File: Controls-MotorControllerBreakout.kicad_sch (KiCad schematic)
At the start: 12 parts, among them J1 MC CAN 1, J2 MC CAN 2, J3 CTRLS, J4 EXT PWR, J5 CANDAPTER

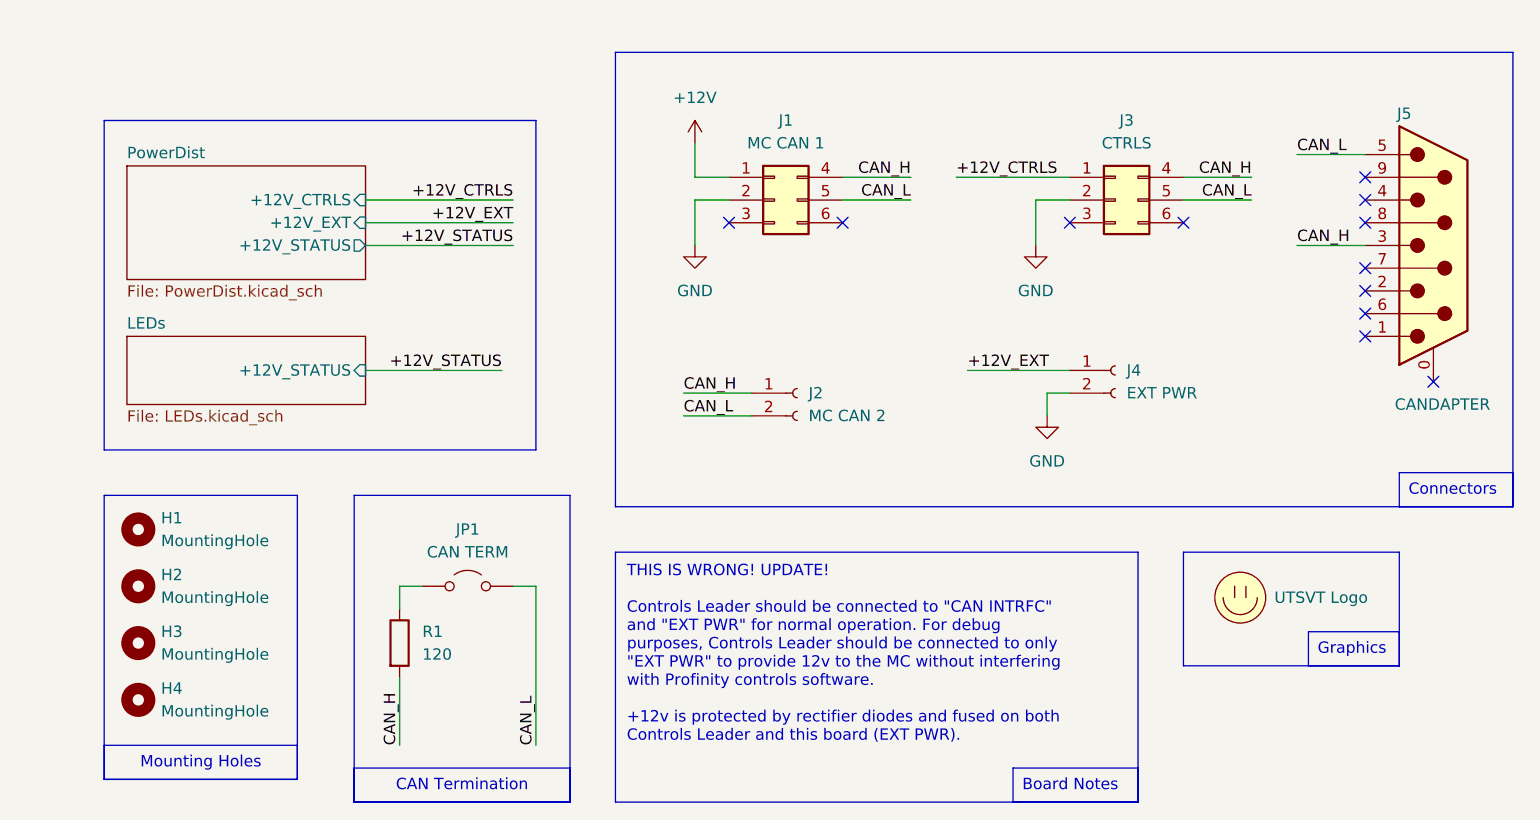
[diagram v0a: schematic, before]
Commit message: layout kinda screwy but it works?
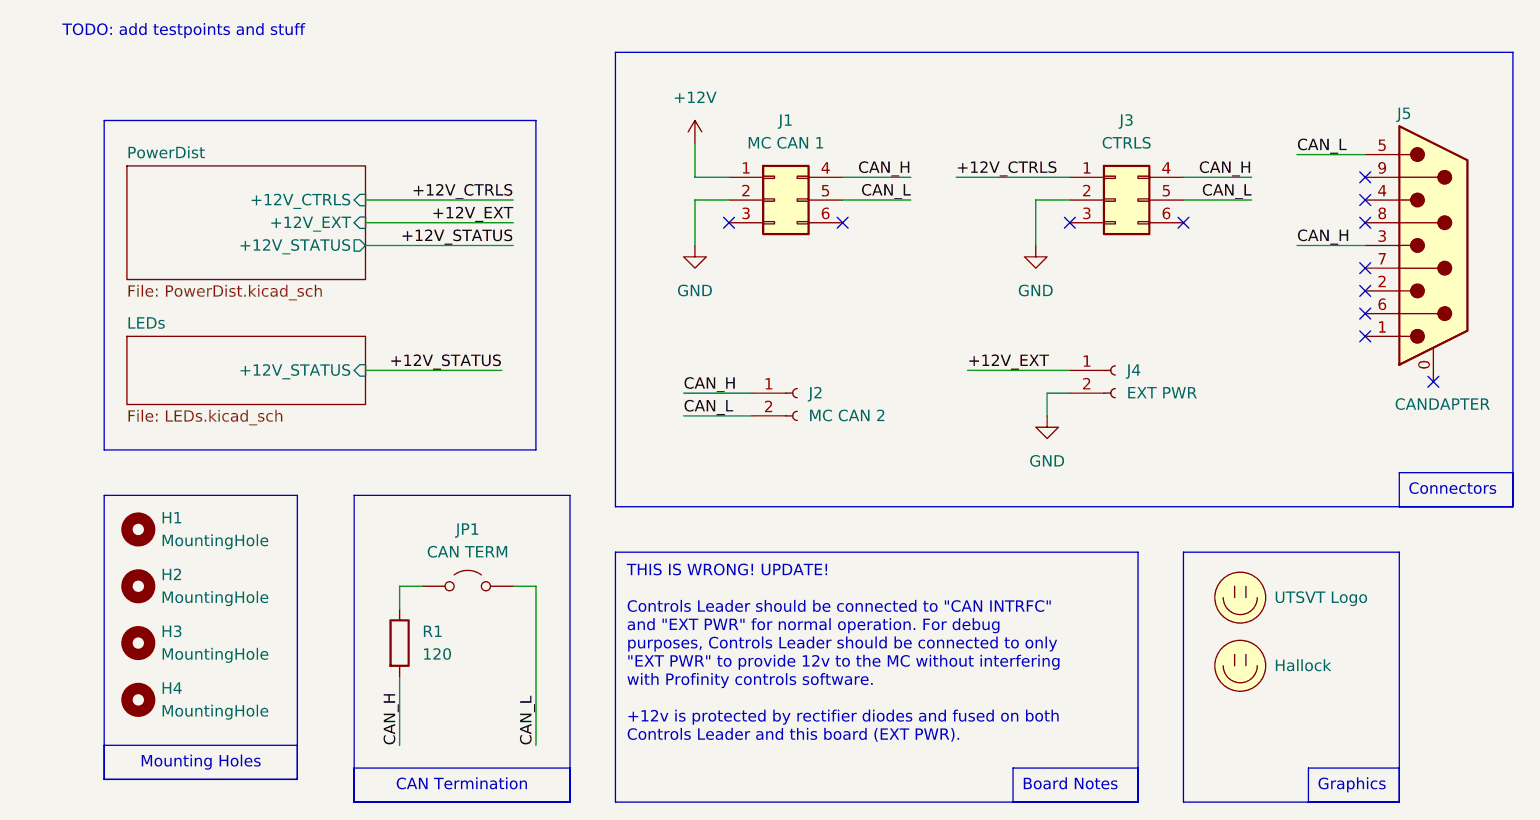
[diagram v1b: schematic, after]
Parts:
- added LOGO2: Hallock, UTSVT_Special:Hallock_Image_Tiny, symbol utsvt-misc:Logo_Placeholder
- H1, H2, H3, H4: footprint (none) -> MountingHole:MountingHole_3mm
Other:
- note added: "TODO: add testpoints and stuff"
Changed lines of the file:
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@@
 	(rectangle
 		(start 140.97 73.66)
-		(end 165.1 86.36)
+		(end 165.1 101.6)
 		(stroke
 			(width 0)
@@
 	(text_box "Graphics"
 		(exclude_from_sim no)
-		(at 154.94 82.55 0)
+		(at 154.94 97.79 0)
 		(size 10.16 3.81)
 		(stroke
@@
 			)
 			(justify top)
+		)
+	)
+	(text "TODO: add testpoints and stuff"
+		(exclude_from_sim no)
+		(at 29.21 15.494 0)
+		(effects
+			(font
+				(size 1.27 1.27)
+			)
 		)
 	)
@@
 			)
 		)
-		(property "Footprint" ""
+		(property "Footprint" "MountingHole:MountingHole_3mm"
 			(at 24.13 83.82 0)
 			(effects
@@
 				(path "/0a971d65-5373-49c6-bc07-3a5d4263dbef"
 					(reference "H3")
+					(unit 1)
+				)
+			)
+		)
+	)
+	(symbol
+		(lib_id "utsvt-misc:Logo_Placeholder")
+		(at 147.32 86.36 0)
+		(unit 1)
+		(exclude_from_sim no)
+		(in_bom yes)
+		(on_board yes)
+		(dnp no)
+		(fields_autoplaced yes)
+		(property "Reference" "LOGO2"
+			(at 147.32 82.55 0)
+			(effects
+				(font
+					(size 1.27 1.27)
+				)
+				(hide yes)
+			)
+		)
+		(property "Value" "Hallock"
+			(at 151.13 86.3599 0)
+			(effects
+				(font
+					(size 1.27 1.27)
+				)
+				(justify left)
+			)
+		)
+		(property "Footprint" "UTSVT_Special:Hallock_Image_Tiny"
+			(at 147.32 84.455 0)
+			(effects
+				(font
+					(size 1.27 1.27)
+				)
+				(hide yes)
+			)
+		)
+		(property "Datasheet" ""
+			(at 147.32 84.455 0)
+			(effects
+				(font
+					(size 1.27 1.27)
+				)
+				(hide yes)
+			)
+		)
+		(property "Description" "Graph footprint placeholder"
+			(at 147.32 86.36 0)
+			(effects
+				(font
+					(size 1.27 1.27)
+				)
+				(hide yes)
+			)
+		)
+		(instances
+			(project ""
+				(path "/0a971d65-5373-49c6-bc07-3a5d4263dbef"
+					(reference "LOGO2")
 					(unit 1)
 				)
@@
 			)
 		)
-		(property "Footprint" ""
+		(property "Footprint" "MountingHole:MountingHole_3mm"
 			(at 24.13 71.12 0)
 			(effects
@@
 			)
 		)
-		(property "Datasheet" "~"
+		(property "Datasheet" "https://cdn.amphenol-cs.com/media/wysiwyg/files/drawing/l77sdxxxsa4ch3r.pdf"
 			(at 168.91 39.37 0)
 			(effects
@@
 			)
 		)
-		(property "Footprint" ""
+		(property "Footprint" "MountingHole:MountingHole_3mm"
 			(at 24.13 77.47 0)
 			(effects
@@
 			)
 		)
-		(property "Footprint" ""
+		(property "Footprint" "MountingHole:MountingHole_3mm"
 			(at 24.13 90.17 0)
 			(effects
